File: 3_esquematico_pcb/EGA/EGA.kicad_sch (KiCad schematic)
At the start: 39 parts, among them J1 12V, J10 TEST_TRIG, J11 POTENCIOMETRO, J2 HC-SR04, J3 LCD 20x4, J4 RTC, J5 TEST_PWM, J6 FAN_12V_PWM_3.3V, J7 UART, J8 TEST_RPM, J9 TEST_ECHO, SW1 PAGINA, SW2 RESET, U1 LM7805_TO220, U2 LM317_TO-220, U3 Pico

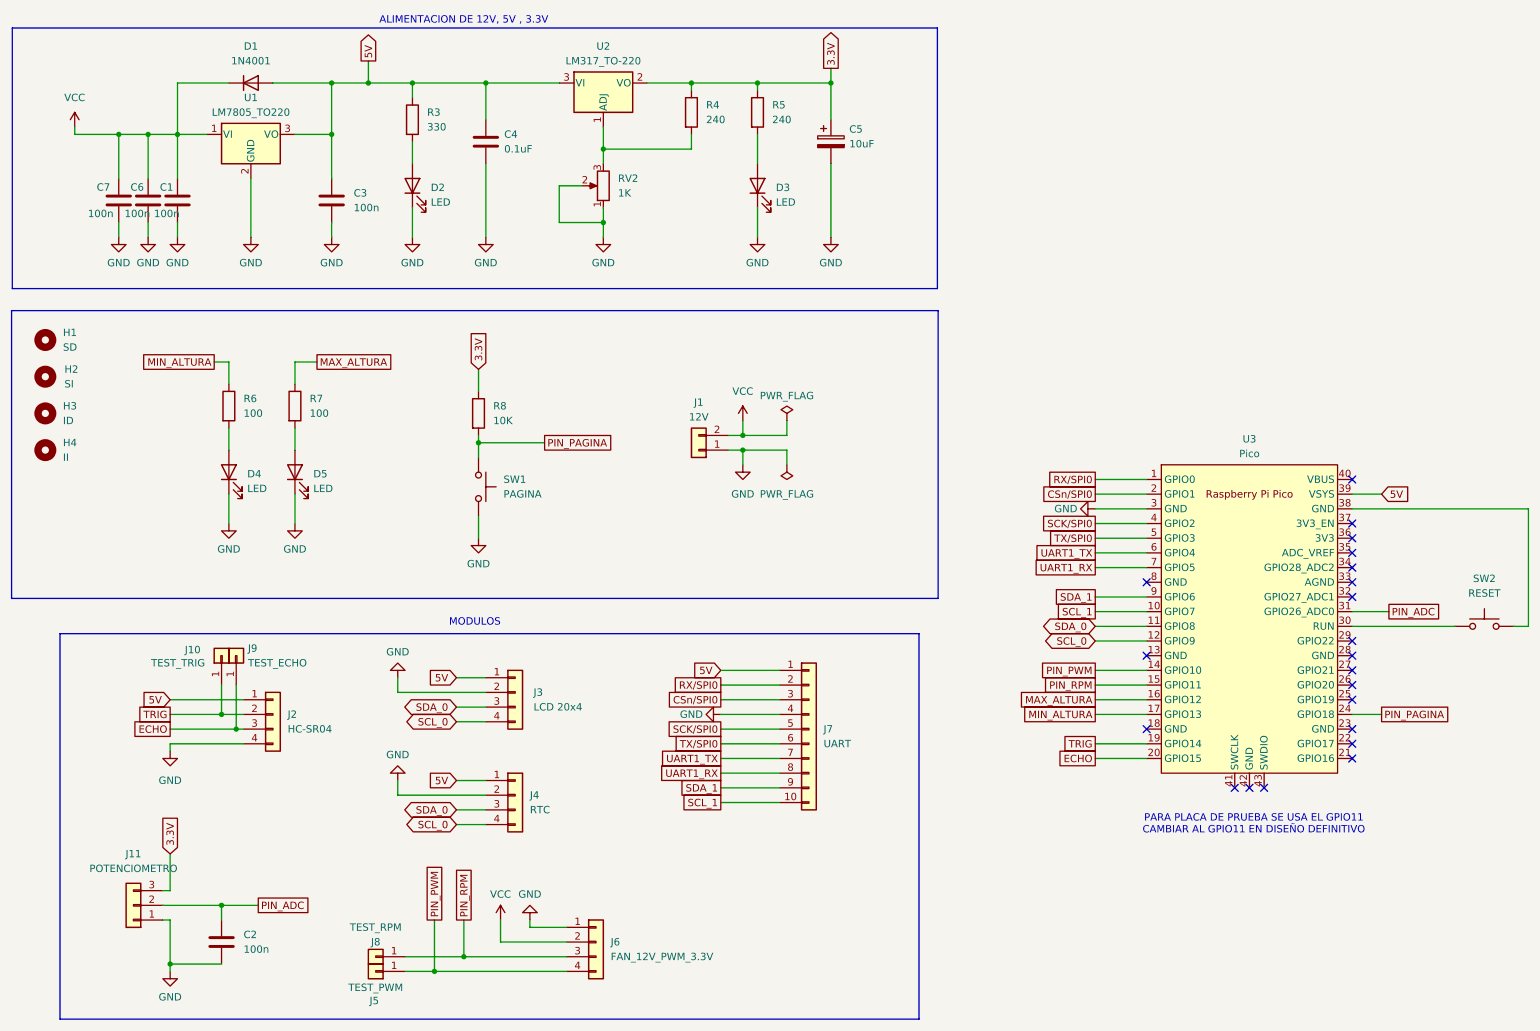
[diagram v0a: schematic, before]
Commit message: Actualizacion 10/12/2025
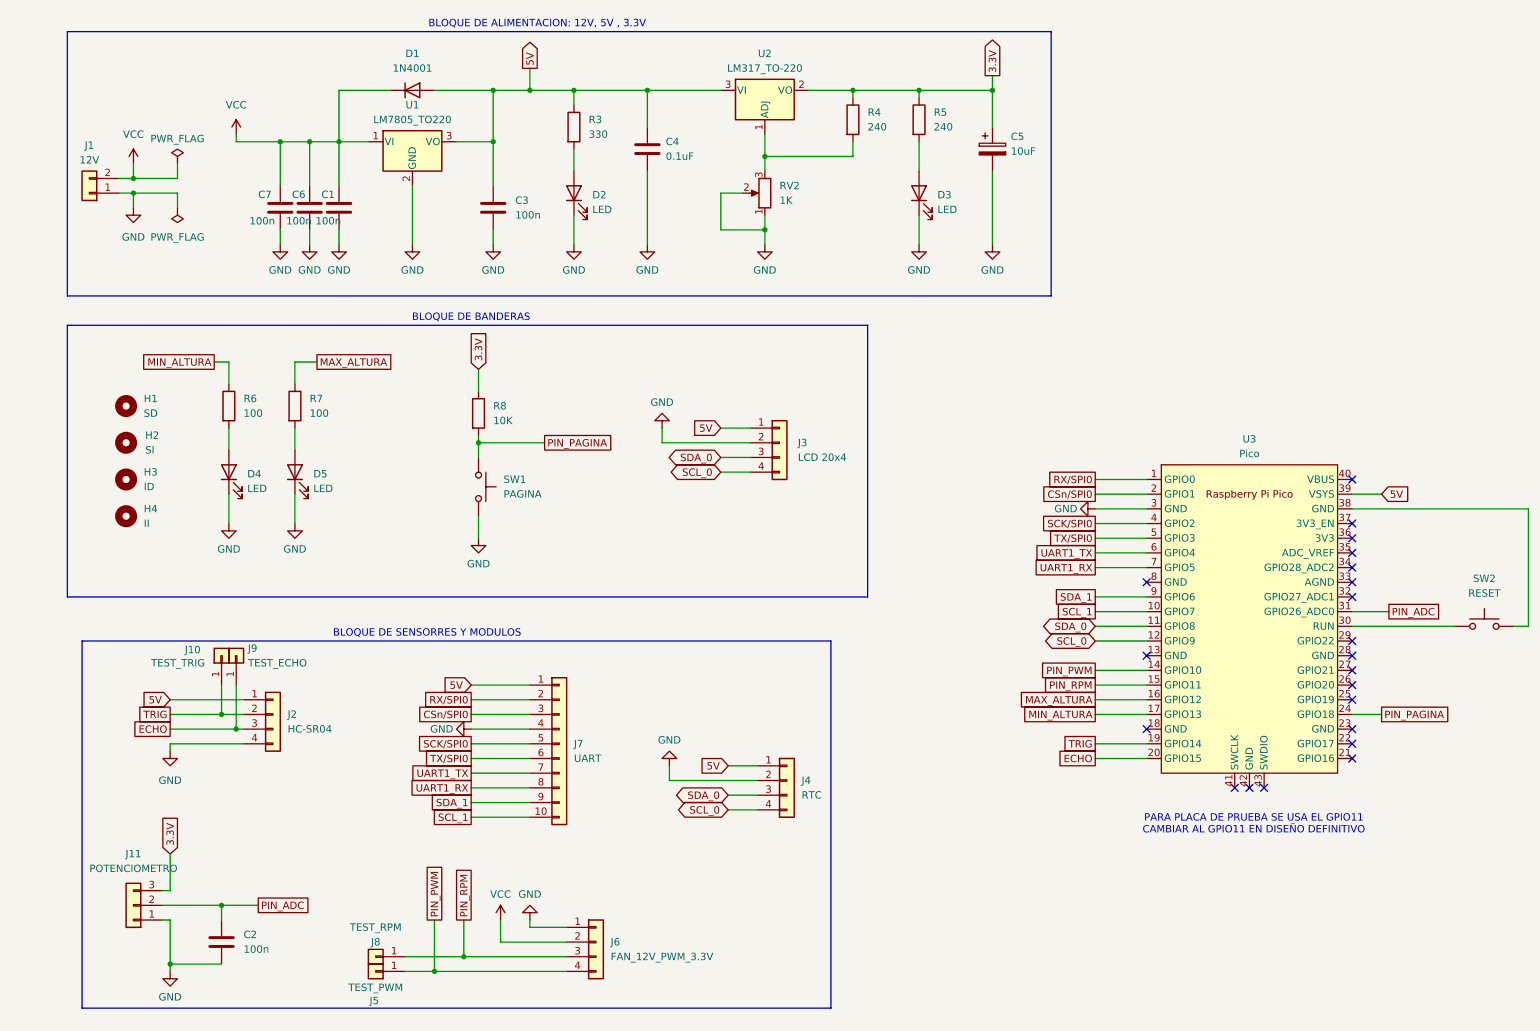
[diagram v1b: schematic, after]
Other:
- note added: "BLOQUE DE ALIMENTACION: 12V, 5V , 3.3V"
- note added: "BLOQUE DE BANDERAS"
- note added: "BLOQUE DE SENSORRES Y MODULOS"
- note removed: "ALIMENTACION DE 12V, 5V , 3.3V"
- note removed: "MODULOS"
- moved on the sheet: C1, C3, C4, C5, C6, C7, D1, D2, D3, H1, H2, H3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
